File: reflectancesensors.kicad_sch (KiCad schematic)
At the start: 17 parts, among them J1 Conn_01x04_Pin, Q1 BPW40, Q2 BPW40, U1 TCRT5000L, U3 TCRT5000L

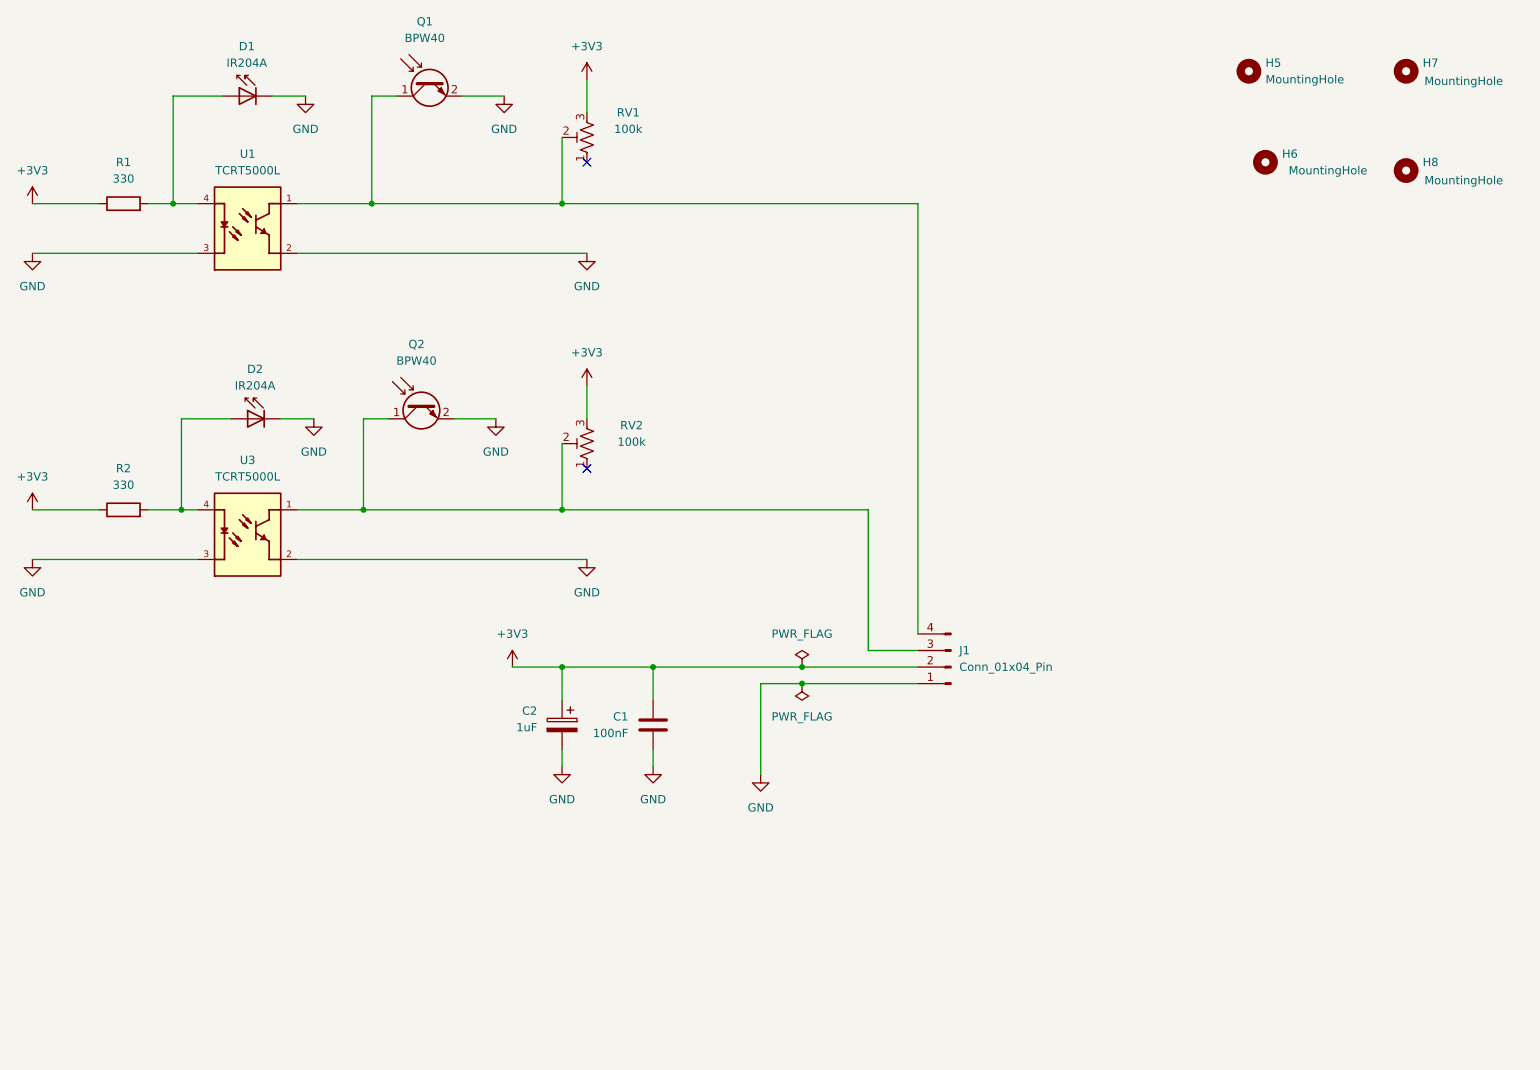
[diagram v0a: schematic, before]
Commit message: changing connector
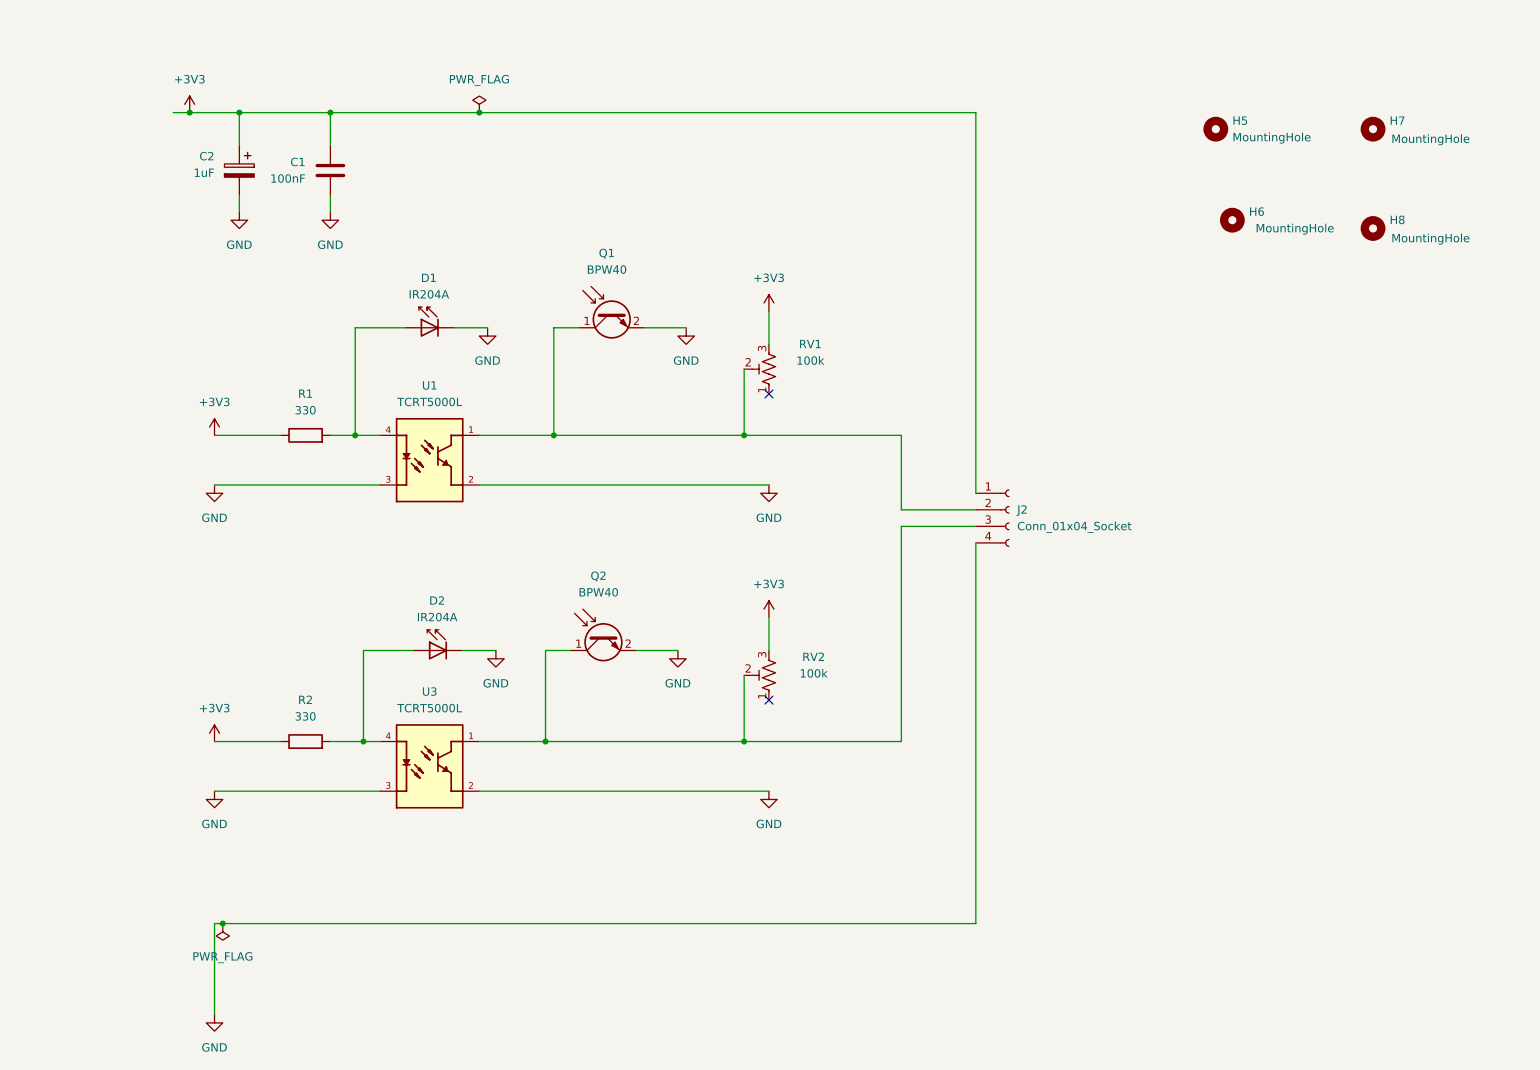
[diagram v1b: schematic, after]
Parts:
- removed J1: Conn_01x04_Pin, Connector_JST:JST_EH_S4B-EH_1x04_P2.50mm_Horizontal, symbol Connector:Conn_01x04_Pin
- added J2: Conn_01x04_Socket, Connector_JST:JST_XH_S4B-XH-A-1_1x04_P2.50mm_Horizontal, symbol Connector:Conn_01x04_Socket
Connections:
- net +3V3: now also J2.1 (Pin_1)
- net GND: now also J2.4 (Pin_4)
- net at Q1.1 (C), RV1.2, U1.1: now also J2.2 (Pin_2)
- net at Q2.1 (C), RV2.2, U3.1: now also J2.3 (Pin_3)
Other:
- moved on the sheet: C1, C2, D1, D2, H5, H6, H7, H8, Q1, Q2, R1, R2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
